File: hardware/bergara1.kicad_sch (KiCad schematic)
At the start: 10 parts, among them J1 Screw_Terminal_01x02, SW1 SW_Nidec_CAS-120A1, U1 TA6586, U2 TA6586, U3 LM7805_TO220, U4 ESP32-C3_SUPERMINI_TH

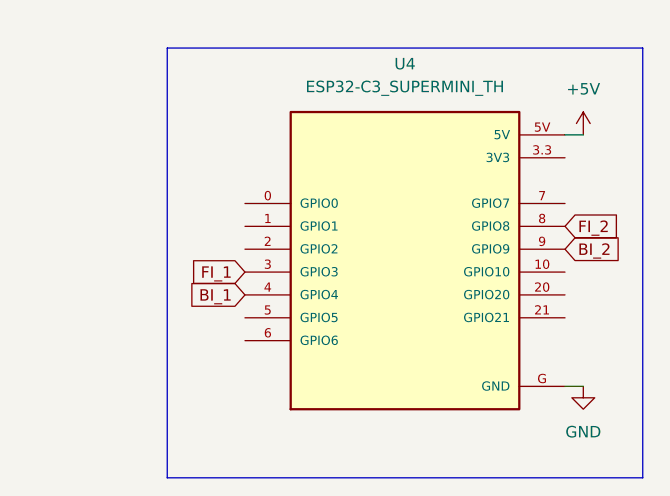
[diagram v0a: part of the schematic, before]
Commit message: Hola
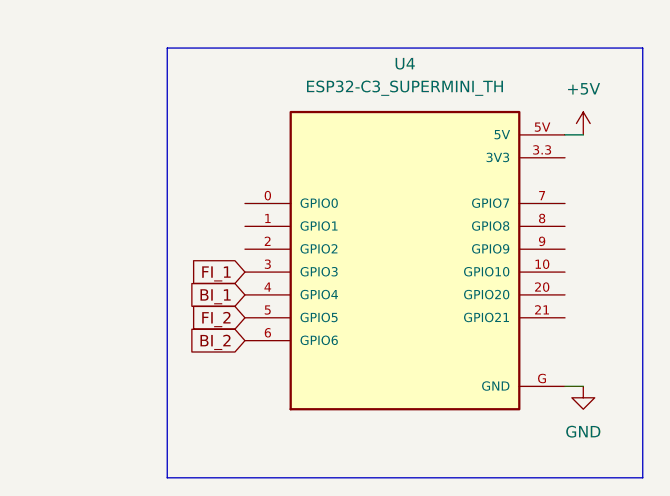
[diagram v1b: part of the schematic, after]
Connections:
- net BI_2: now also U4.6 (GPIO6); no longer U4.9 (GPIO9)
- net FI_2: now also U4.5 (GPIO5); no longer U4.8 (GPIO8)
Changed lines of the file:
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@@
+		)
+	)
+	(global_label "FI_2"
+		(shape input)
+		(at 46.736 173.228 180)
+		(fields_autoplaced yes)
+		(effects
+			(font
+				(size 1.27 1.27)
+			)
+			(justify right)
+		)
+		(property "Intersheetrefs" "${INTERSHEET_REFS}"
+			(at 39.8803 173.228 0)
+			(effects
+				(font
+					(size 1.27 1.27)
+				)
+				(justify right)
+				(hide yes)
+			)
+		)
+	)
+	(global_label "BI_2"
+		(shape input)
+		(at 46.736 175.768 180)
+		(fields_autoplaced yes)
+		(effects
+			(font
+				(size 1.27 1.27)
+			)
+			(justify right)
+		)
+		(property "Intersheetrefs" "${INTERSHEET_REFS}"
+			(at 39.6989 175.768 0)
+			(effects
+				(font
+					(size 1.27 1.27)
+				)
+				(justify right)
+				(hide yes)
+			)
 		)
 	)
@@
 		)
 	)
-	(global_label "BI_2"
-		(shape input)
-		(at 82.296 165.608 0)
-		(fields_autoplaced yes)
-		(effects
-			(font
-				(size 1.27 1.27)
-			)
-			(justify left)
-		)
-		(property "Intersheetrefs" "${INTERSHEET_REFS}"
-			(at 89.3331 165.608 0)
-			(effects
-				(font
-					(size 1.27 1.27)
-				)
-				(justify left)
-				(hide yes)
-			)
-		)
-	)
 	(global_label "FI_1"
 		(shape input)
@@
 				(hide yes)
 			)
-		)
-	)
-	(global_label "FI_2"
-		(shape input)
-		(at 82.296 163.068 0)
-		(fields_autoplaced yes)
-		(effects
-			(font
-				(size 1.27 1.27)
-			)
-			(justify left)
-		)
-		(property "Intersheetrefs" "${INTERSHEET_REFS}"
-			(at 89.1517 163.068 0)
-			(effects
-				(font
-					(size 1.27 1.27)
-				)
-				(justify left)
-				(hide yes)
-			)
